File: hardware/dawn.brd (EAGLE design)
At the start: 68.2 x 68.6 mm, 33 parts, among them IC1 ATMEGA328-20P, IC3 DS1307, Q2 16Mhz, Q3 32.768kHz, Q4 BUZ11BV, T3 BC547B, T4 BC547B, X1 MKDSN1,5/2-5,08, X2 MKDSN1,5/2-5,08

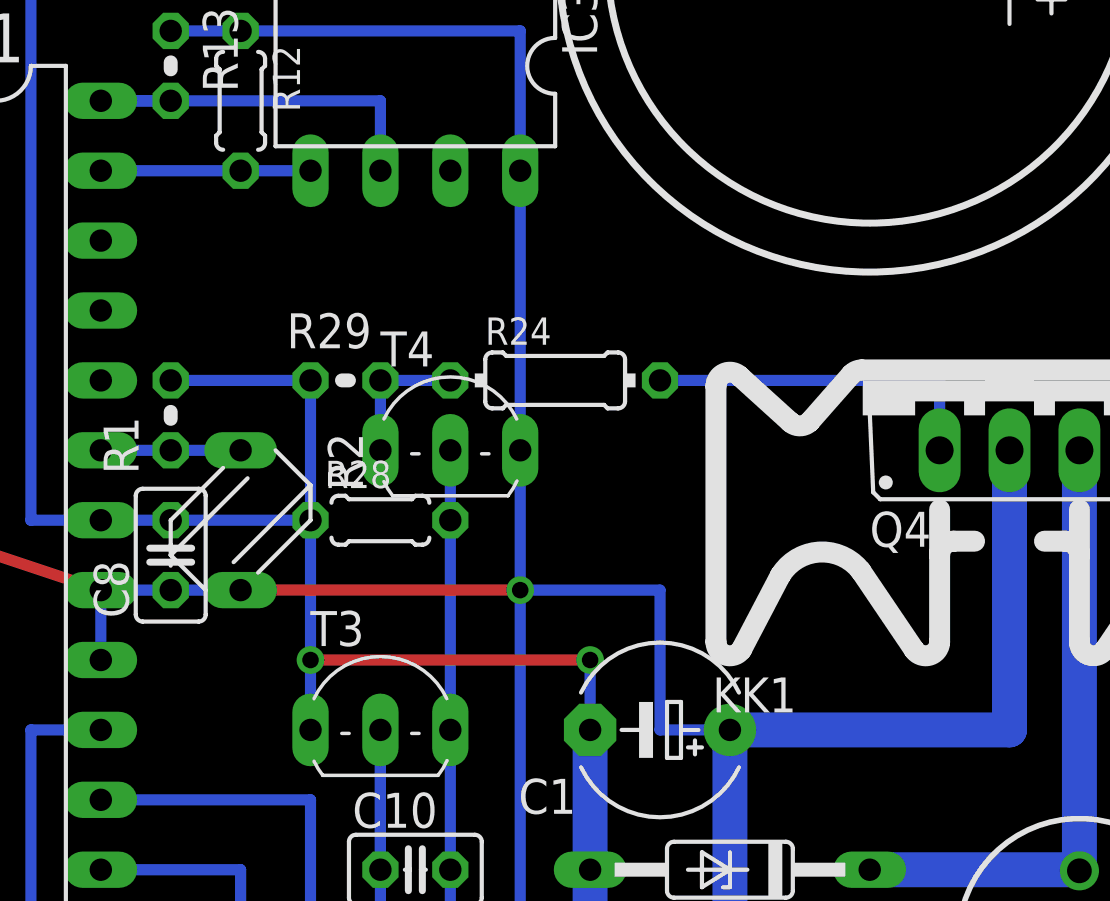
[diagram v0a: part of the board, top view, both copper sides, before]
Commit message: Cleanup
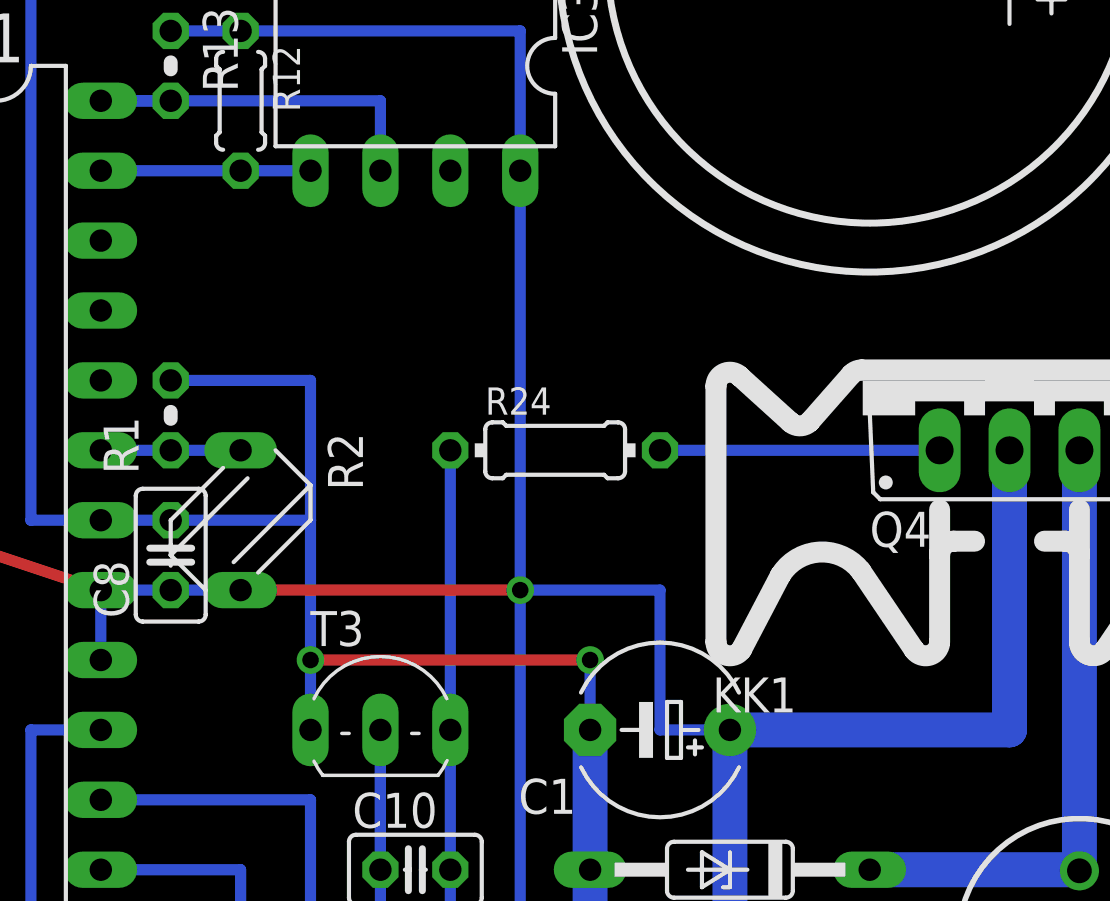
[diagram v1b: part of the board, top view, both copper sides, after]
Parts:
- removed R28: 1k, rcl:0204/5
- removed R29: 10k, rcl:0204V
- removed T4: BC547B, transistor-neu-to92:TO92-EBC
- moved R24 2.54 mm to (69.8, 49.5)
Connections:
- removed net N$43: R24.1, R29.2, T4.E
- net +5V: no longer T4.C
- net GND: no longer R28.1, R29.1
- net N$41: now also R24.1; no longer R28.2, T4.B
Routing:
- net N$43: track 5.08 -> 0.00 mm
- net N$37: track 12.7 -> 10.2 mm
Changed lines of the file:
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@@
 <element name="R13" library="rcl" package="0204V" value="10k" x="55.88" y="63.5" rot="R270"/>
 <element name="U$1" library="jy-mcu" package="JY-MCU" value="JY-MCU" x="38.1" y="55.88" rot="R180"/>
-<element name="R24" library="rcl" package="0204/7" value="10" x="69.85" y="52.07"/>
+<element name="R24" library="rcl" package="0204/7" value="10" x="69.85" y="49.53"/>
 <element name="Q4" library="transistor-power" package="TO220BV" value="BUZ11BV" x="86.36" y="52.07"/>
 <element name="R25" library="rcl" package="0411/12" value="1W" x="77.47" y="29.21"/>
@@
 <element name="C10" library="rcl" package="C025-025X050" value="100pF" x="64.77" y="34.29"/>
 <element name="R27" library="rcl" package="0207/10" value="4.7k" x="60.96" y="29.21"/>
-<element name="R28" library="rcl" package="0204/5" value="1k" x="63.5" y="46.99"/>
-<element name="T4" library="transistor-neu-to92" package="TO92-EBC" value="BC547B" x="66.04" y="50.8"/>
-<element name="R29" library="rcl" package="0204V" value="10k" x="62.23" y="52.07"/>
 <element name="X1" library="con-phoenix-508" package="MKDSN1,5/2-5,08" value="MKDSN1,5/2-5,08" x="73.66" y="21.59"/>
 <element name="X2" library="con-phoenix-508" package="MKDSN1,5/2-5,08" value="MKDSN1,5/2-5,08" x="86.36" y="21.59"/>
@@
 <contactref element="C9" pad="1"/>
 <contactref element="U$1" pad="VCC"/>
-<contactref element="T4" pad="C"/>
-<wire x1="68.58" y1="49.53" x2="68.58" y2="59.69" width="0.4064" layer="16"/>
 <wire x1="38.1" y1="52.07" x2="43.18" y2="52.07" width="0.4064" layer="16"/>
 <wire x1="68.58" y1="64.77" x2="58.42" y2="64.77" width="0.4064" layer="16"/>
@@
 <wire x1="76.1789" y1="21.615" x2="76.2" y2="21.615" width="1.27" layer="16"/>
 <wire x1="86.36" y1="49.53" x2="86.36" y2="44.45" width="1.27" layer="16"/>
-<wire x1="68.58" y1="49.53" x2="68.58" y2="44.45" width="0.4064" layer="16"/>
 <wire x1="86.36" y1="49.53" x2="86.36" y2="39.37" width="1.27" layer="16"/>
 <wire x1="86.36" y1="39.37" x2="76.2" y2="39.37" width="1.27" layer="16"/>
@@
 <wire x1="53.34" y1="21.59" x2="68.58" y2="21.59" width="0.4064" layer="16"/>
 <wire x1="68.58" y1="21.59" x2="68.58" y2="22.86" width="0.4064" layer="16"/>
+<wire x1="68.58" y1="44.45" x2="68.58" y2="59.69" width="0.4064" layer="16"/>
 </signal>
 <signal name="GND">
@@
 <contactref element="T3" pad="E"/>
 <contactref element="R25" pad="1"/>
-<contactref element="R28" pad="1"/>
-<contactref element="R29" pad="1"/>
 <wire x1="71.12" y1="34.29" x2="71.12" y2="29.21" width="1.27" layer="16"/>
 <wire x1="71.12" y1="29.21" x2="71.12" y2="24.155" width="1.27" layer="16"/>
@@
 <contactref element="IC1" pad="22"/>
 <contactref element="X1" pad="1"/>
-<wire x1="60.96" y1="41.91" x2="60.96" y2="46.99" width="0.4064" layer="16"/>
 <wire x1="71.0989" y1="21.615" x2="71.12" y2="24.155" width="1.27" layer="16"/>
 <wire x1="71.12" y1="24.155" x2="71.12" y2="24.13" width="1.27" layer="16"/>
@@
 <wire x1="60.96" y1="41.91" x2="71.12" y2="41.91" width="0.4064" layer="1"/>
 <via x="71.12" y="41.91" extent="1-16" drill="0.6" shape="square"/>
-<wire x1="60.96" y1="52.07" x2="60.96" y2="46.99" width="0.4064" layer="16"/>
 <wire x1="53.34" y1="46.99" x2="50.8" y2="46.99" width="0.4064" layer="16"/>
 <contactref element="JP1" pad="1"/>
@@
 <wire x1="40.64" y1="44.45" x2="40.64" y2="46.99" width="0.4064" layer="16"/>
 <wire x1="53.34" y1="46.99" x2="55.88" y2="46.99" width="0.4064" layer="16"/>
-<wire x1="55.88" y1="46.99" x2="60.96" y2="46.99" width="0.4064" layer="16"/>
 <wire x1="50.8" y1="46.99" x2="50.8" y2="67.31" width="0.4064" layer="16"/>
 <wire x1="50.8" y1="67.31" x2="33.02" y2="67.31" width="0.4064" layer="16"/>
@@
 <wire x1="71.12" y1="34.29" x2="71.12" y2="39.37" width="1.27" layer="16"/>
 <wire x1="71.12" y1="39.37" x2="71.12" y2="41.91" width="0.4064" layer="16"/>
-<wire x1="55.88" y1="52.07" x2="60.96" y2="52.07" width="0.4064" layer="16"/>
 <contactref element="U$2" pad="GND"/>
 <wire x1="40.64" y1="21.59" x2="48.26" y2="21.59" width="0.4064" layer="16"/>
+<wire x1="60.96" y1="41.91" x2="60.96" y2="46.99" width="0.4064" layer="16"/>
+<wire x1="60.96" y1="46.99" x2="55.88" y2="46.99" width="0.4064" layer="16"/>
+<wire x1="55.88" y1="52.07" x2="60.96" y2="52.07" width="0.4064" layer="16"/>
+<wire x1="60.96" y1="52.07" x2="60.96" y2="46.99" width="0.4064" layer="16"/>
 </signal>
 <signal name="N$13">
@@
 <contactref element="Q4" pad="G"/>
 <contactref element="R24" pad="2"/>
-<wire x1="83.82" y1="52.07" x2="73.66" y2="52.07" width="0.4064" layer="16"/>
-<wire x1="83.82" y1="49.53" x2="83.82" y2="52.07" width="0.4064" layer="16"/>
+<wire x1="83.82" y1="49.53" x2="73.66" y2="49.53" width="0.4064" layer="16"/>
 </signal>
 <signal name="N$39">
@@
 <contactref element="C10" pad="2"/>
 <contactref element="T3" pad="C"/>
-<contactref element="T4" pad="B"/>
-<contactref element="R28" pad="2"/>
 <contactref element="R27" pad="2"/>
-<wire x1="66.04" y1="49.53" x2="66.04" y2="46.99" width="0.4064" layer="16"/>
 <wire x1="66.04" y1="29.21" x2="66.04" y2="34.29" width="0.4064" layer="16"/>
 <wire x1="66.04" y1="39.37" x2="66.04" y2="34.29" width="0.4064" layer="16"/>
-<wire x1="66.04" y1="46.99" x2="66.04" y2="39.37" width="0.4064" layer="16"/>
-</signal>
-<signal name="N$43">
 <contactref element="R24" pad="1"/>
-<contactref element="R29" pad="2"/>
-<contactref element="T4" pad="E"/>
-<wire x1="63.5" y1="49.53" x2="63.5" y2="52.07" width="0.4064" layer="16"/>
-<wire x1="63.5" y1="52.07" x2="66.04" y2="52.07" width="0.4064" layer="16"/>
+<wire x1="66.04" y1="39.37" x2="66.04" y2="49.53" width="0.4064" layer="16"/>
 </signal>
 <signal name="N$2">
